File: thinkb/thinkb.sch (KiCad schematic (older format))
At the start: 128 parts, among them SW1 SW_Push, SW14 SW_Push, SW15 SW_Push, SW16 SW_Push, SW17 SW_Push, SW18 SW_Push, SW19 SW_Push, SW2 SW_Push, SW20 SW_Push, SW25 SW_Push, SW26 SW_Push, SW27 SW_Push, SW28 SW_Push, SW29 SW_Push, SW3 SW_Push, SW30 SW_Push, SW31 SW_Push, SW32 SW_Push, SW37 SW_Push, SW38 SW_Push, SW39 SW_Push, SW4 SW_Push, SW40 SW_Push, SW41 SW_Push, SW42 SW_Push, SW43 SW_Push, SW44 SW_Push, SW49 SW_Push, SW5 SW_Push, SW50 SW_Push, SW51 SW_Push, SW52 SW_Push, SW53 SW_Push, SW54 SW_Push, SW55 SW_Push, SW56 SW_Push, SW6 SW_Push, SW7 SW_Push, SW8 SW_Push, SW9 SW_Push, U1 ProMicro_2

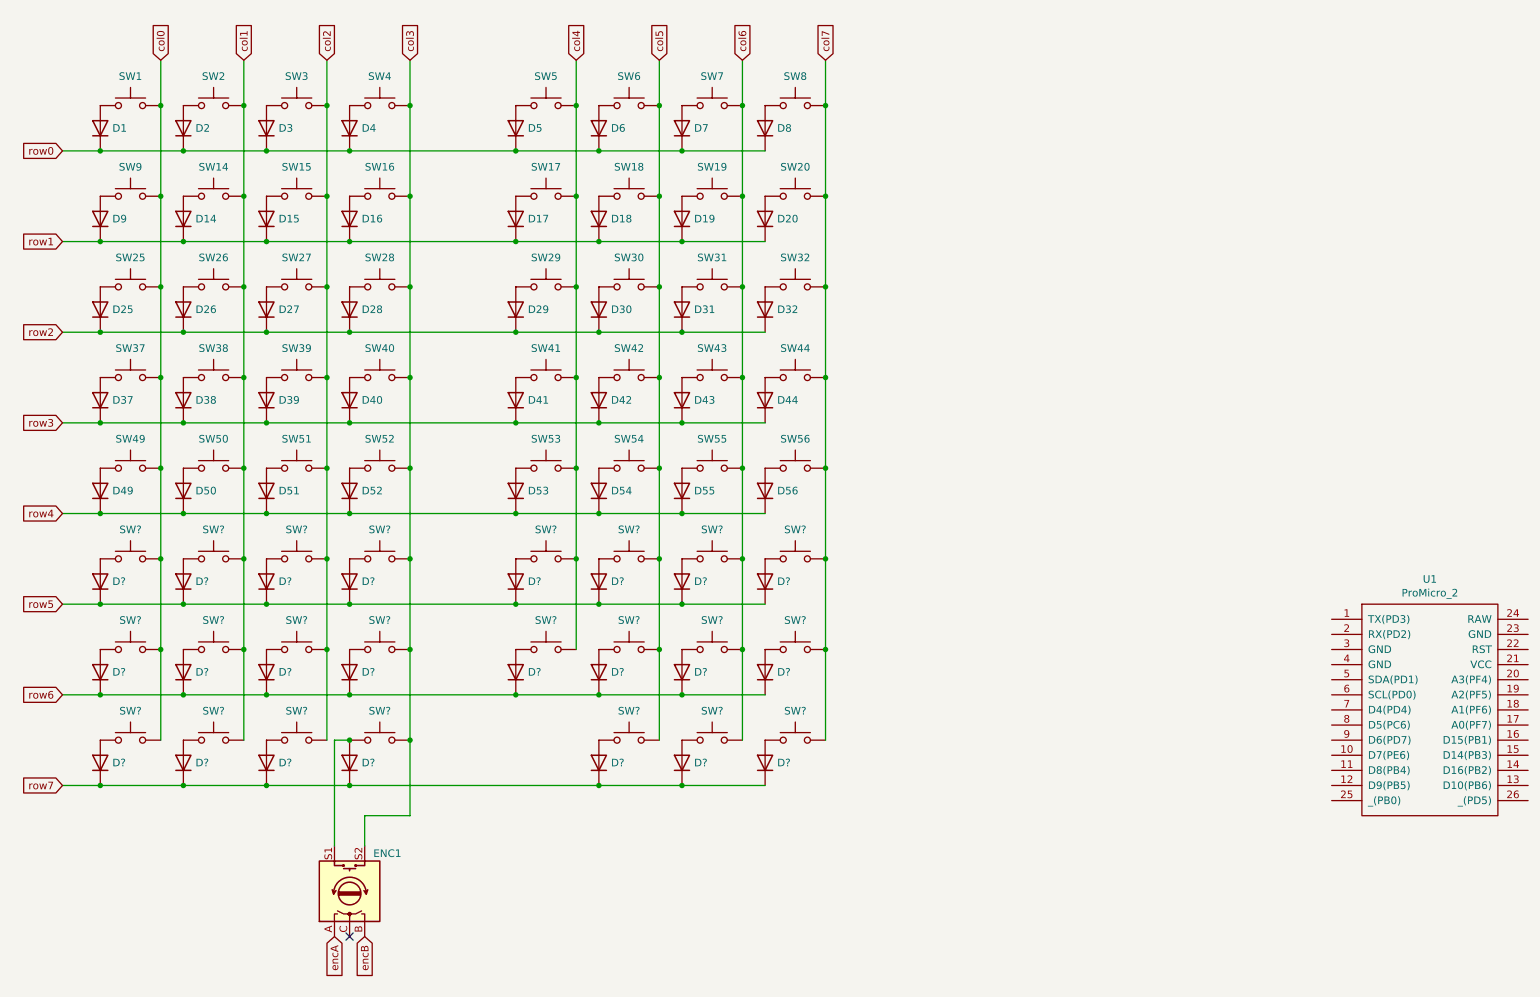
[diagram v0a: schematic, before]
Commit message: WIP on keyboard matrix
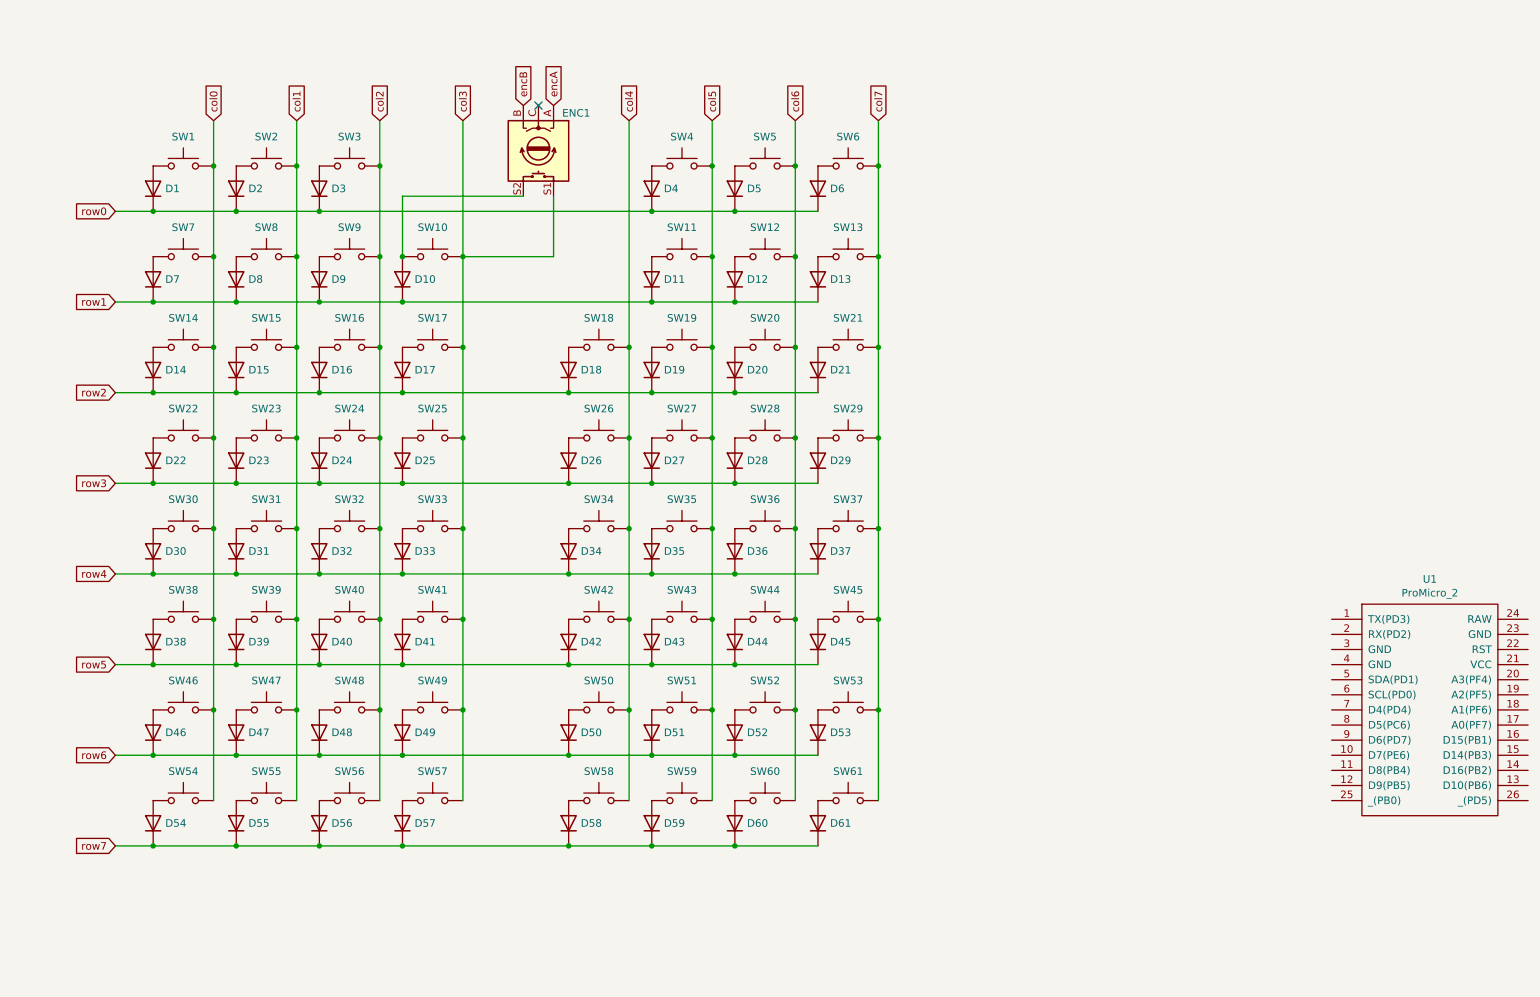
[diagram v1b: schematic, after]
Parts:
- removed D17, D4, D5: 1N4148, footprints:diode_TH_SMD, symbol Diode:1N4148
- removed SW17, SW4, SW5: SW_Push, footprints:Choc_PG1350_Choc_Spacing, symbol Switch:SW_Push
- added D58: 1N4148, footprints:diode_TH_SMD, symbol Diode:1N4148
- added SW58: SW_Push, footprints:Choc_PG1350_Choc_Spacing, symbol Switch:SW_Push
- gave numbers to parts that had none: 46
- renumbered D16 to D10, D18 to D11, D19 to D12, D20 to D13, D25 to D14, D26 to D15, D27 to D16, D28 to D17, D29 to D18, D30 to D19, D31 to D20, D32 to D21, D37 to D22, D38 to D23, D39 to D24, D40 to D25, D41 to D26, D42 to D27, D43 to D28, D44 to D29, D49 to D30, D50 to D31, D51 to D32, D52 to D33, D53 to D34, D54 to D35, D55 to D36, D56 to D37, D6 to D4, D7 to D5, D8 to D6, D9 to D7, D14 to D8, D15 to D9, SW16 to SW10, SW18 to SW11, SW19 to SW12, SW20 to SW13, SW25 to SW14, SW26 to SW15, SW27 to SW16, SW28 to SW17, SW29 to SW18, SW30 to SW19, SW31 to SW20, SW32 to SW21, SW37 to SW22, SW38 to SW23, SW39 to SW24, SW40 to SW25, SW41 to SW26, SW42 to SW27, SW43 to SW28, SW44 to SW29, SW49 to SW30, SW50 to SW31, SW51 to SW32, SW52 to SW33, SW53 to SW34, SW54 to SW35, SW55 to SW36, SW56 to SW37, SW6 to SW4, SW7 to SW5, SW8 to SW6, SW9 to SW7, SW14 to SW8, SW15 to SW9
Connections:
- net col3: now also ENC1.S1; no longer ENC1.S2
- net col4: now also SW58.2
- net row7: now also D58.1 (K)
- net at D10.2 (A), SW10.1: now also ENC1.S2
- net at D57.2 (A), SW57.1: no longer ENC1.S1
- new net: D58.2 (A), SW58.1
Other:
- moved on the sheet: D1, D10, D11, D12, D13, D14, D15, D16, D17, D18, D19, D2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
